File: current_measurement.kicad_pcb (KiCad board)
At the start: 2 copper layers, 30 x 19.3 mm, 15 parts, among them J1 Conn_01x02_Male, J2 Conn_01x02_Female, J3 Conn_01x02_Male, J4 USB_B_Micro, U1 MAX680CSA+T, U2 INA105

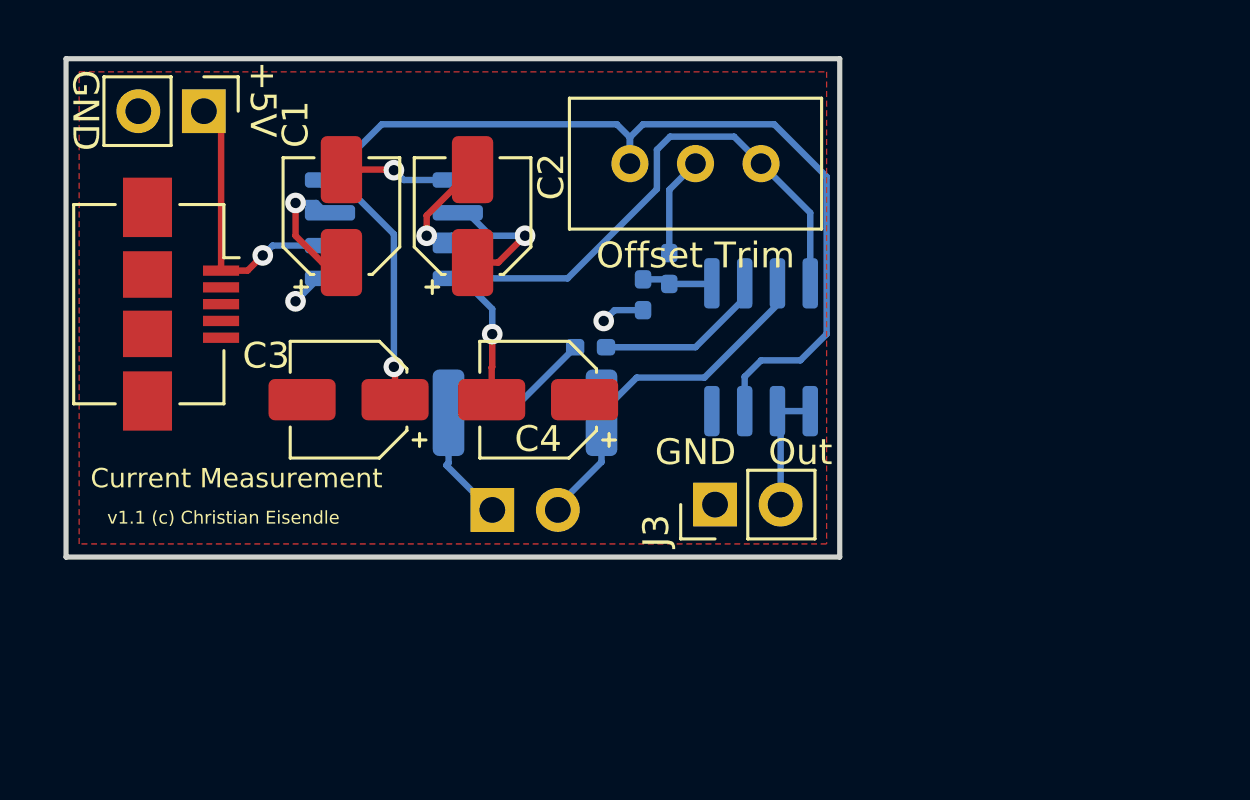
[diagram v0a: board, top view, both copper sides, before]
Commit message: Current Shunt 2.0
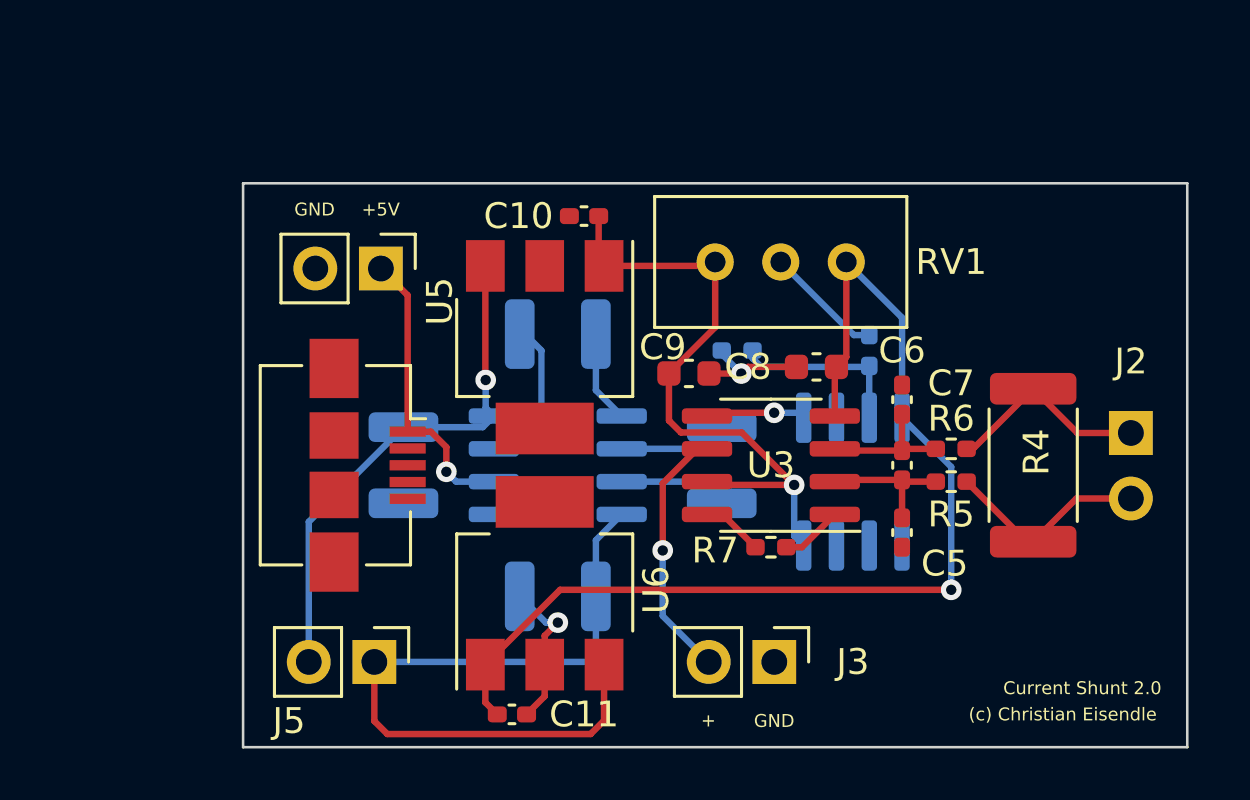
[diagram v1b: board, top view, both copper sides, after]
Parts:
- removed R1: 10, Resistor_SMD:R_0402_1005Metric_Pad0.72x0.64mm_HandSolder
- removed U2: INA105, Package_SO:SOIC-8_3.9x4.9mm_P1.27mm
- added C10: 1u, Capacitor_SMD:C_0402_1005Metric_Pad0.74x0.62mm_HandSolder, F.Cu at (106.4, 61.5)
- added C11: 1u, Capacitor_SMD:C_0402_1005Metric_Pad0.74x0.62mm_HandSolder, F.Cu at (103.6, 80.8)
- added C5: 1n, Capacitor_SMD:C_0402_1005Metric_Pad0.74x0.62mm_HandSolder, F.Cu at (118.7, 73.7)
- added C6: 1n, Capacitor_SMD:C_0402_1005Metric_Pad0.74x0.62mm_HandSolder, F.Cu at (118.7, 68.6)
- added C7: 47n, Capacitor_SMD:C_0402_1005Metric_Pad0.74x0.62mm_HandSolder, F.Cu at (118.7, 71.1)
- added C8: 100n, Capacitor_SMD:C_0603_1608Metric, F.Cu at (115.4, 67.3)
- added C9: 100n, Capacitor_SMD:C_0603_1608Metric, F.Cu at (110.5, 67.6)
- added J5: DualSupp, Connector_PinHeader_2.54mm:PinHeader_1x02_P2.54mm_Vertical, F.Cu at (98.3, 78.7)
- added R5: 4k02, Resistor_SMD:R_0402_1005Metric_Pad0.72x0.64mm_HandSolder, F.Cu at (120.7, 71.8)
- added R6: 4k02, Resistor_SMD:R_0402_1005Metric_Pad0.72x0.64mm_HandSolder, F.Cu at (120.7, 70.5)
- added R7: 845, Resistor_SMD:R_0402_1005Metric_Pad0.72x0.64mm_HandSolder, F.Cu at (113.7, 74.3)
- added U3: AD620, Package_SO:SOIC-8_3.9x4.9mm_P1.27mm, F.Cu at (113.7, 71.1)
- added U4: OPA2277, Package_SO:SOIC-8_3.9x4.9mm_P1.27mm, B.Cu at (116.8, 71.8)
- added U5: XC6216D802FR-G, Package_TO_SOT_SMD:SOT-223-3_TabPin2, F.Cu at (104.9, 66.5)
- added U6: XC6902N801PR-G, Package_TO_SOT_SMD:SOT-223-3_TabPin2, F.Cu at (104.9, 75.7)
- C1, C2, C3, C4: footprint Capacitor_SMD:CP_Elec_4x5.8 -> Capacitor_SMD:C_1210_3225Metric; moved to B.Cu
- R4: moved to F.Cu
- moved J2 24.9 mm to (127.6, 69.9), turned to 180 degrees
- moved R4 19.8 mm to (123.8, 71.1), turned to 90 degrees
- moved C2 13.6 mm to (111.8, 71.1), turned to -90 degrees
- moved U1 11.1 mm to (105.4, 71.1)
- moved J4 9.55 mm to (98.0, 71.1)
- moved C1 9.55 mm to (105.4, 66.0), turned to 0 degrees
- moved J1 9.18 mm to (98.6, 63.5)
- moved R3 8.37 mm to (117.5, 66.7)
- moved C4 7.66 mm to (105.4, 76.2), turned to 0 degrees
- moved J3 6.51 mm to (113.8, 78.7), turned to -90 degrees
- moved RV1 5.04 mm to (116.6, 63.2)
- moved R2 4.24 mm to (112.4, 66.7), turned to 0 degrees
- moved C3 3.31 mm to (99.4, 71.1), turned to -90 degrees
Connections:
- C3 pad 1: +10V -> Net-(C3-Pad1)
- C4 pad 2: -10V -> Net-(U1-Pad4)
- U1 pad 4: -10V -> Net-(U1-Pad4)
- U1 pad 8: +10V -> Net-(C3-Pad1)
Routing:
- net Net-(U1-Pad4): track 0.00 -> 28.4 mm
- net Net-(C3-Pad1): track 0.00 -> 20.3 mm, vias 0 -> 1
- net +10V: track 45.1 -> 25.1 mm
- net -10V: track 25.8 -> 41.9 mm
- net GND: track 3.25 -> 10.7 mm
- net Net-(R1-Pad2): track 6.73 -> 0.00 mm
- net Net-(C5-Pad2): track 0.00 -> 5.44 mm
- net Net-(C6-Pad1): track 0.00 -> 5.37 mm
- net Net-(J2-Pad2): track 13.7 -> 8.49 mm
- net Net-(U3-Pad5): track 0.00 -> 5.15 mm, vias 0 -> 1
- net Net-(J3-Pad2): track 4.94 -> 9.92 mm, vias 0 -> 1
- net Net-(R2-Pad2): track 2.75 -> 6.99 mm
- net Net-(J2-Pad1): track 10.5 -> 8.04 mm
- net Net-(R7-Pad2): track 0.00 -> 2.40 mm
- net Net-(R7-Pad1): track 0.00 -> 2.40 mm
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- added copper zone on B.Cu, net GND
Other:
- board size 30 x 19.3 mm -> 36.6 x 21.8 mm
- board text added: "(c) Christian Eisendle"
- board text added: "+"
- board text added: "Current Shunt 2.0"
- board text removed: "Current Measurement"
- board text removed: "IN+"
- board text removed: "IN-"
- board text removed: "Offset Trim"
- board text removed: "Out"
- board text removed: "v1.1 (c) Christian Eisendle"
